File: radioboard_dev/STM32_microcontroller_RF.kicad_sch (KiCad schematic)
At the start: 71 parts, among them U8 BGS13SN8E6327XTSA1, X4 NT2016SF

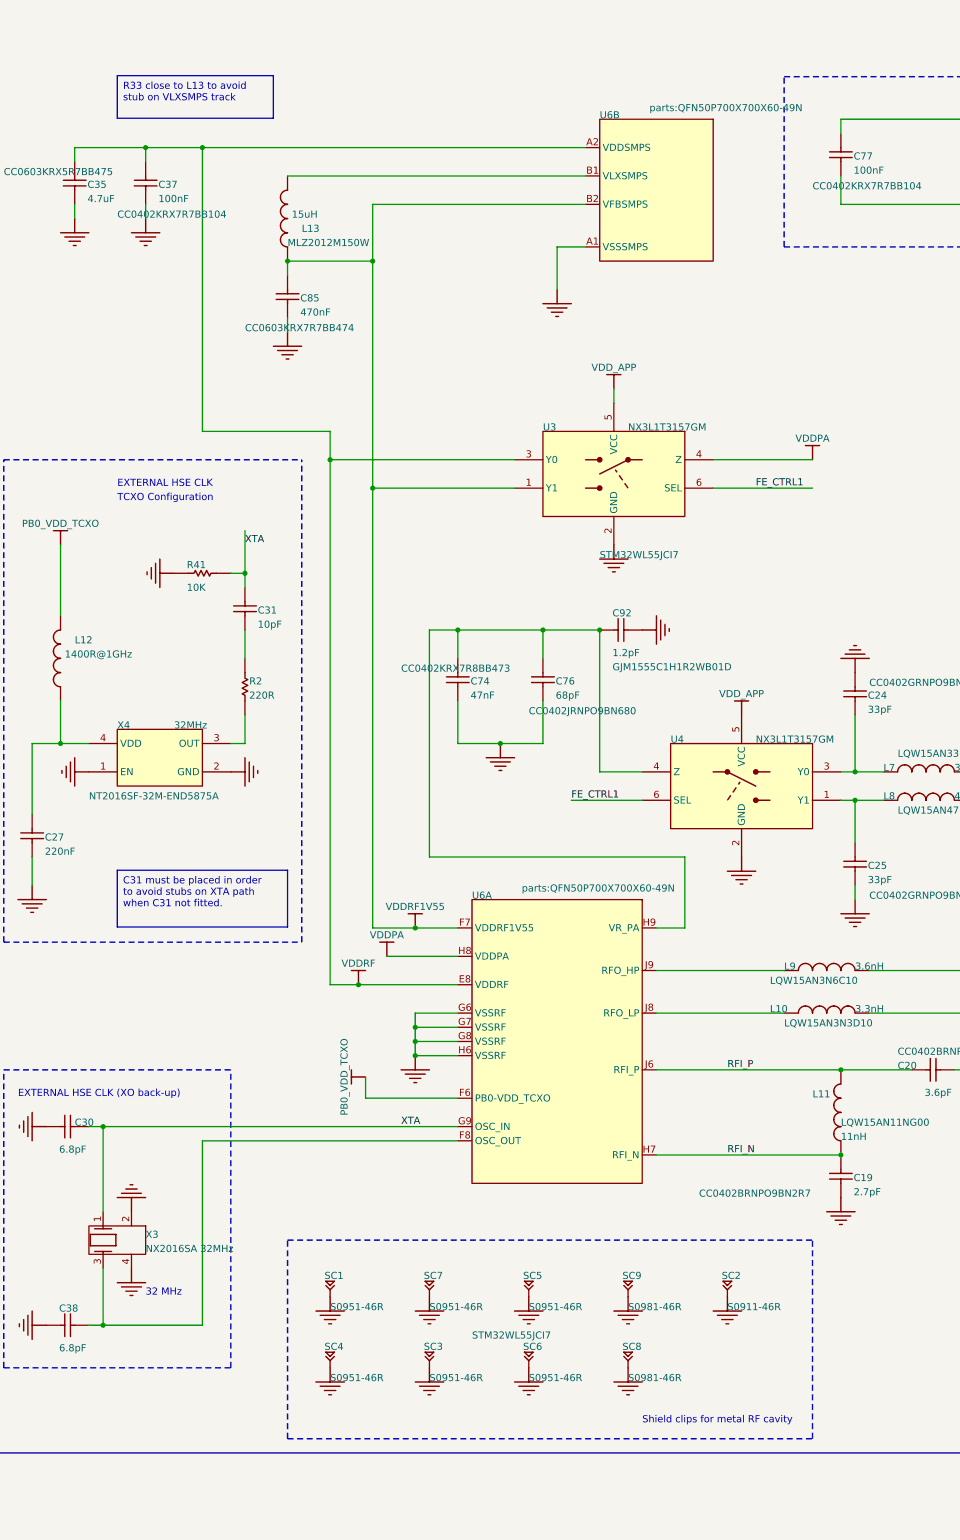
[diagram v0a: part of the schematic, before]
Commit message: finish schematic and clear pcb
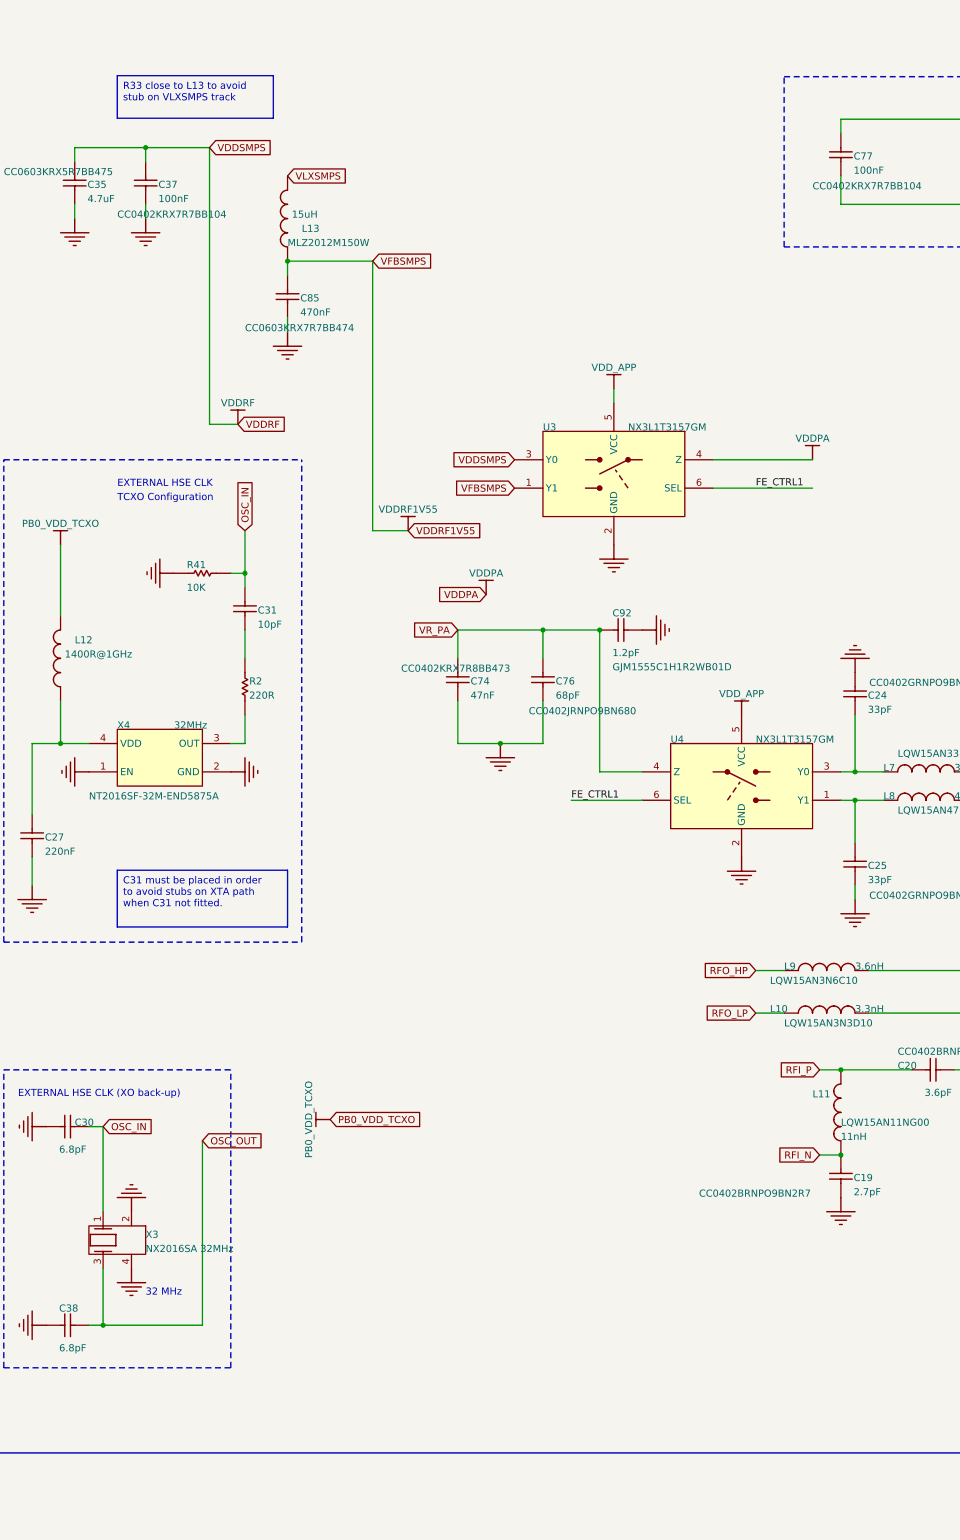
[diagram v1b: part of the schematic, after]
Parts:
- removed SC1, SC3, SC4, SC5, SC6, SC7: ~, CLIP_HARWIN_S0951-46R, symbol MB1389-altium-import:U_STM32_microcontroller_RF_0_Shield-clip_S0951-46R
- removed SC2: Shield-clip_S0951-46R, symbol MB1389-altium-import:U_STM32_microcontroller_RF_0_Shield-clip_S0951-46R
- removed SC8, SC9: Shield-clip_S0981-46R, symbol MB1389-altium-import:U_STM32_microcontroller_RF_0_Shield-clip_S0951-46R
- removed U6: ~, parts:QFN50P700X700X60-49N, symbol MB1389-altium-import:U_STM32_microcontroller_RF_0_STM32WL5x_BGA73
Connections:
- net OSC_OUT: now reaches C38.2, X3.3
- net VLXSMPS: now reaches L13.2
- net RFO_LP: now reaches L10.1
- net VR_PA: now reaches C74.2, C76.2, C92.2, U4.4 (Z)
- net RFO_HP: now reaches L9.1
- net XTA renamed OSC_IN
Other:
- note removed: "Shield clips for metal RF cavity"
